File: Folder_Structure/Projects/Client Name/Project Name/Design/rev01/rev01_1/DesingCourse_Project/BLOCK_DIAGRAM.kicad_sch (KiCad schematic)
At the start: 0 parts

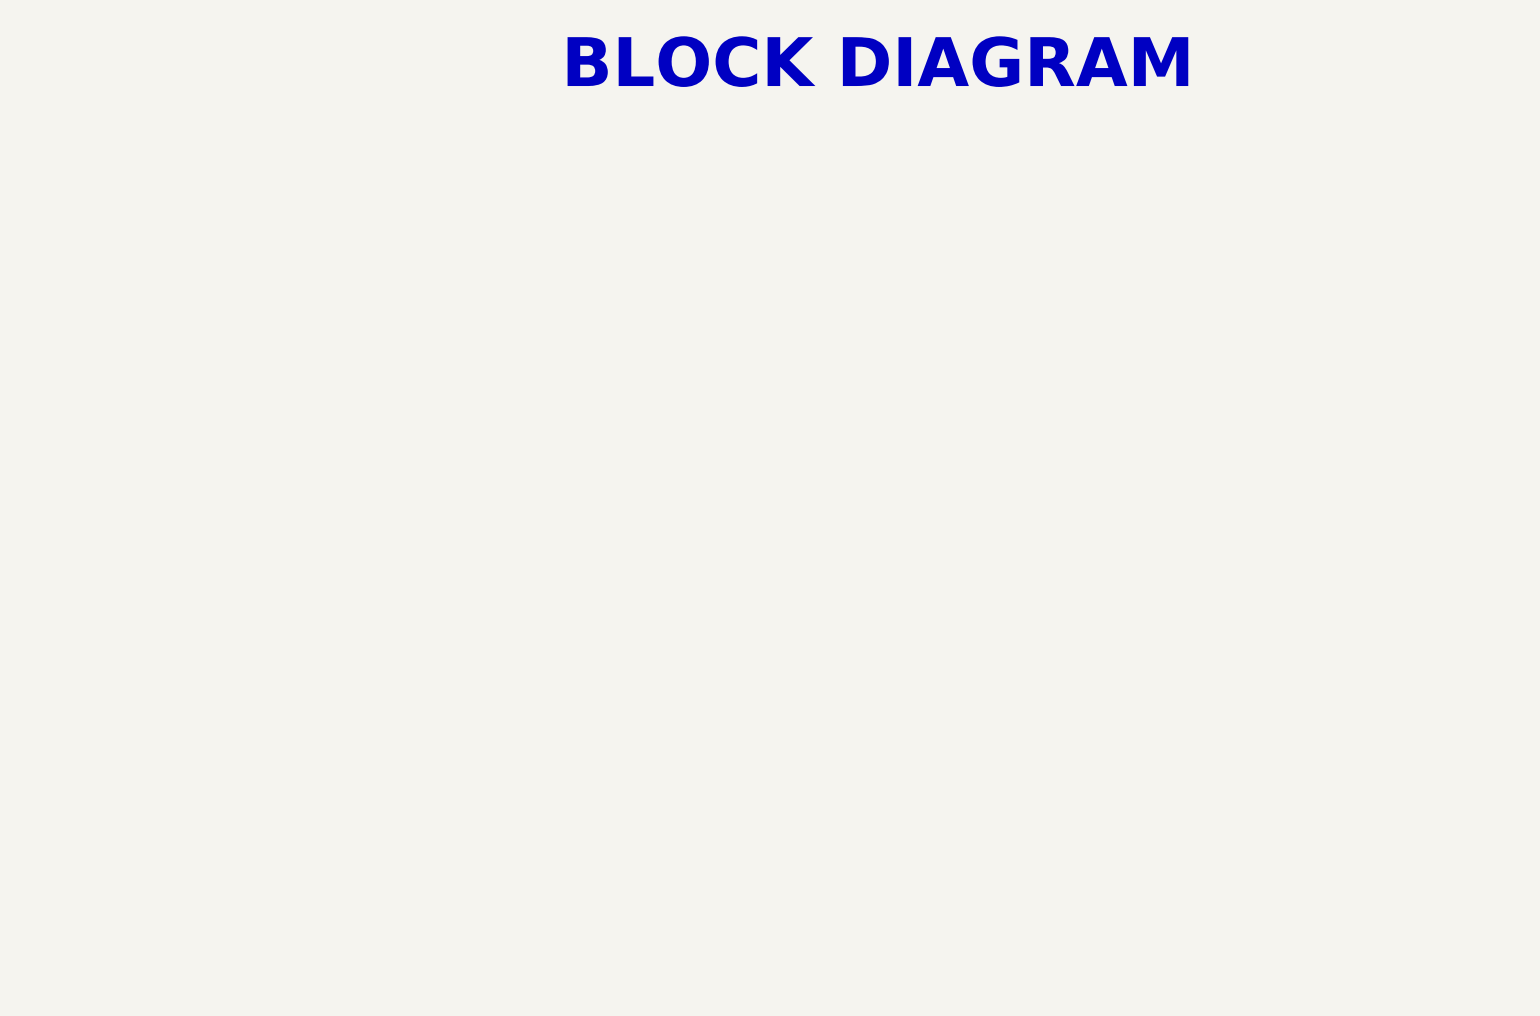
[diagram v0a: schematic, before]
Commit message: Update 15
Ready for DRC
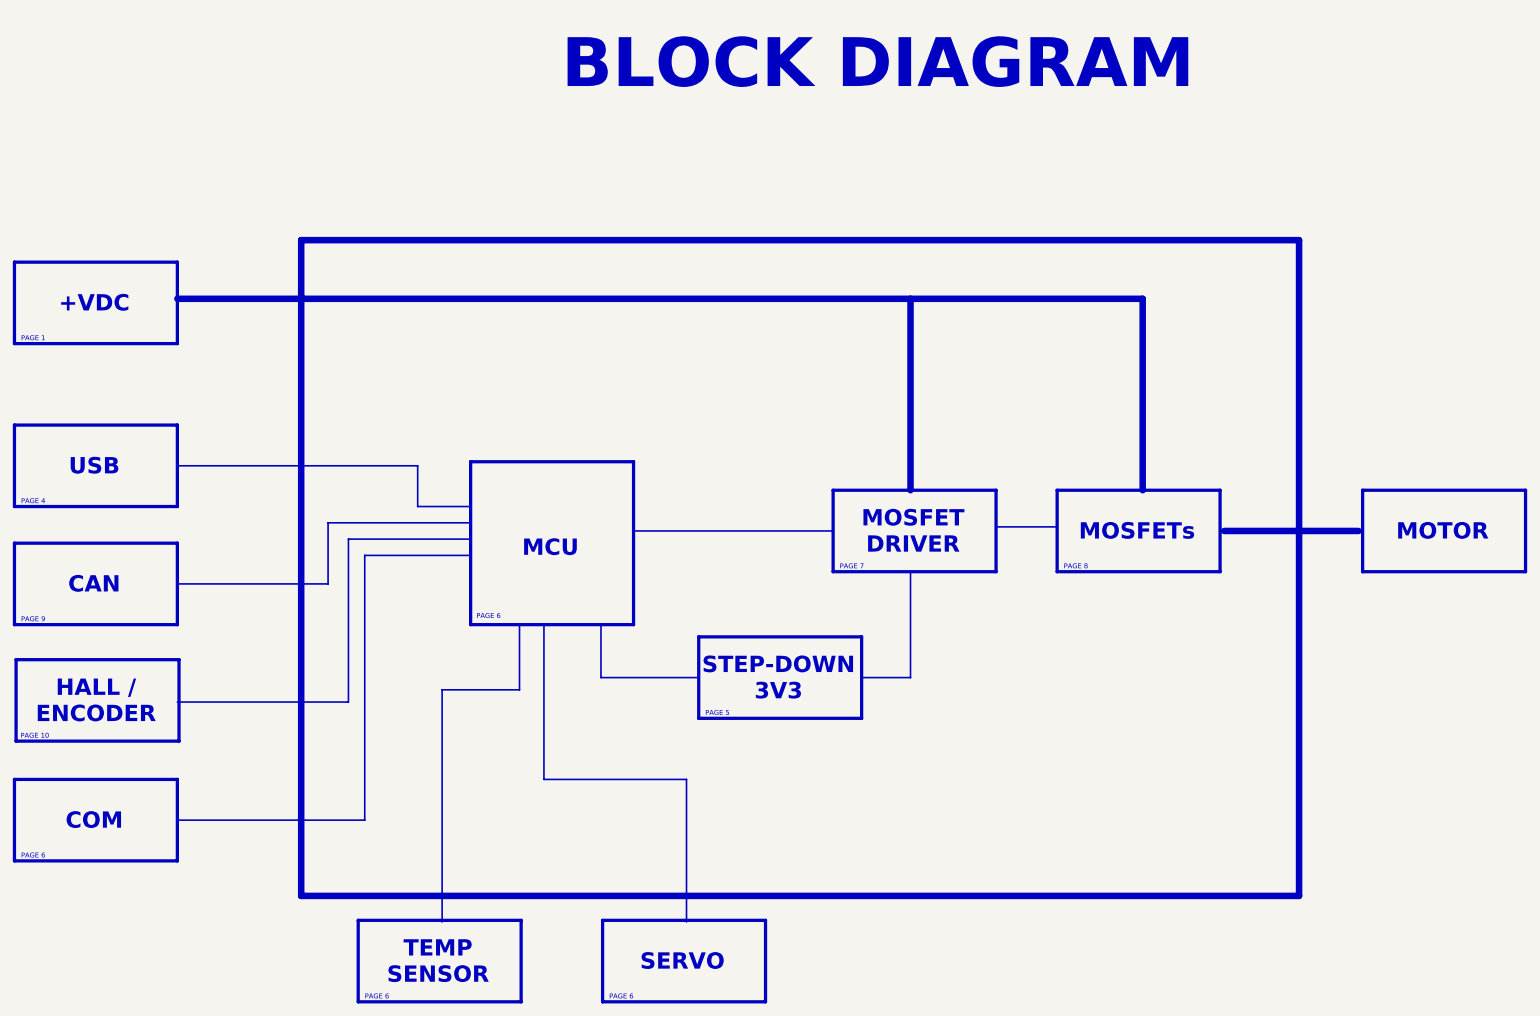
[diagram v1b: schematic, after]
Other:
- note added: "+VDC"
- note added: "CAN"
- note added: "COM"
- note added: "HALL / ENCODER"
- note added: "MCU"
- note added: "MOSFET DRIVER"
- note added: "MOSFETs"
- note added: "MOTOR"
- note added: "PAGE 1"
- note added: "PAGE 10"
- note added: "PAGE 4"
- note added: "PAGE 5"
- note added: "PAGE 6"
- note added: "PAGE 7"
- note added: "PAGE 8"
- note added: "PAGE 9"
- note added: "SERVO"
- note added: "STEP-DOWN 3V3"
- note added: "TEMP SENSOR"
- note added: "USB"
